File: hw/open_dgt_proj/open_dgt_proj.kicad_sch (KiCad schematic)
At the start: 4 parts, among them SW1 SW_Wuerth_450301014042, U1 MiniF4-STM32F401CEU6

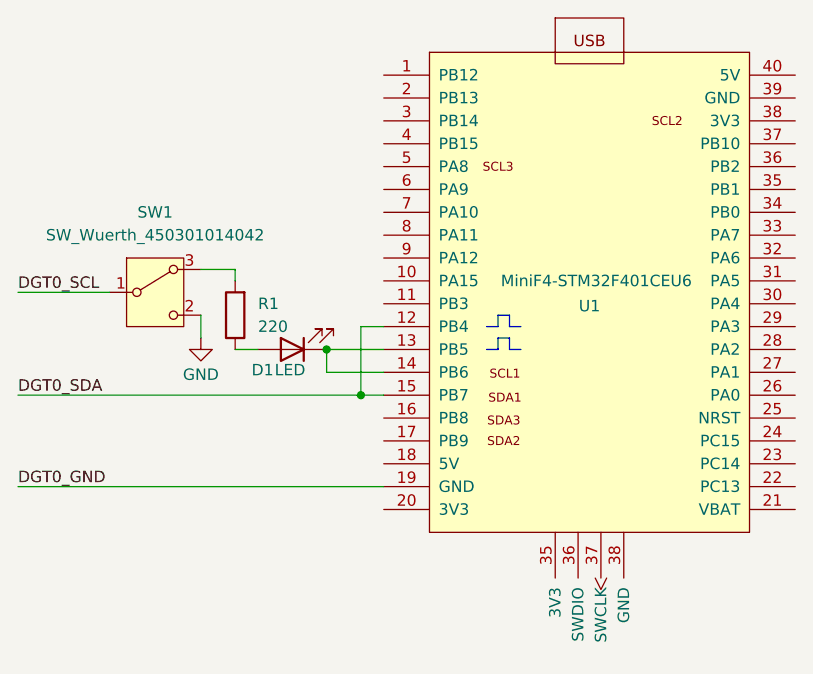
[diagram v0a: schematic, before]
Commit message: Updated project schematic, PCB and 3D model
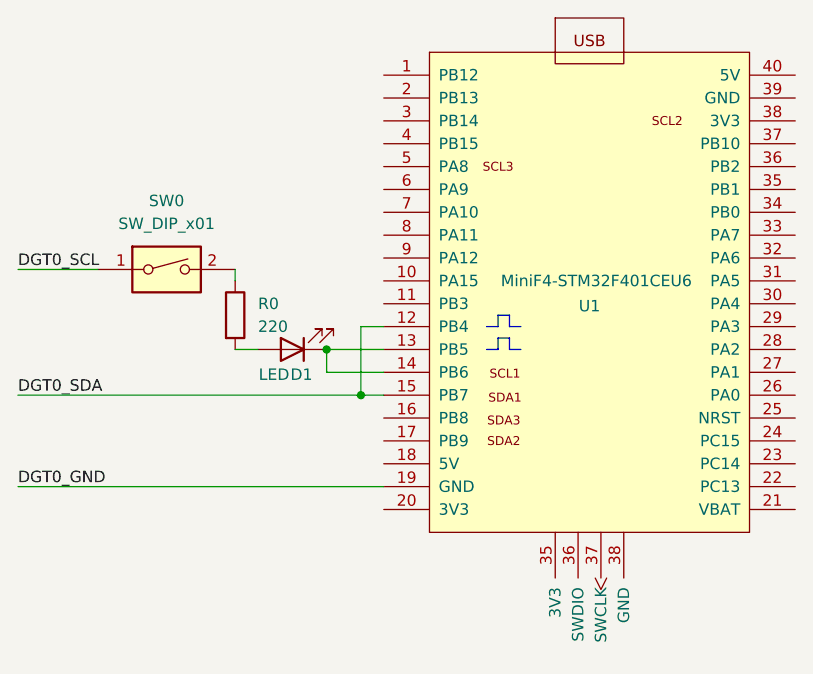
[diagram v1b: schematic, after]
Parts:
- removed R1: 220, symbol Device:R
- removed SW1: SW_Wuerth_450301014042, Button_Switch_THT:SW_Slide-03_Wuerth-WS-SLTV_10x2.5x6.4_P2.54mm, symbol Switch:SW_Wuerth_450301014042
- added R0: 220, Resistor_THT:R_Axial_DIN0207_L6.3mm_D2.5mm_P10.16mm_Horizontal, symbol Device:R
- added SW0: SW_DIP_x01, Button_Switch_THT:SW_DIP_SPSTx01_Slide_6.7x4.1mm_W7.62mm_P2.54mm_LowProfile, symbol Switch:SW_DIP_x01
- D1: footprint (none) -> LED_THT:LED_D5.0mm_FlatTop
- U1: footprint (none) -> BlackPill_v2:YAAJ_BlackPill_SWD_2
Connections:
- net DGT0_SCL: now also SW0.1
- net at D1.2 (A): now also R0.2
- new net: R0.1, SW0.2
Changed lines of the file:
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@@
-	(wire
-		(pts
-			(xy 77.47 83.82) (xy 81.28 83.82)
-		)
-		(stroke
-			(width 0)
-			(type default)
-		)
-	)
 	(wire
 		(pts
@@
 	(wire
 		(pts
-			(xy 77.47 88.9) (xy 77.47 91.44)
-		)
-		(stroke
-			(width 0)
-			(type default)
-		)
-	)
-	(wire
-		(pts
 			(xy 91.44 92.71) (xy 97.79 92.71)
 		)
@@
 	(wire
 		(pts
-			(xy 57.15 86.36) (xy 67.31 86.36)
+			(xy 57.15 83.82) (xy 66.04 83.82)
 		)
 		(stroke
@@
 	)
 	(label "DGT0_SCL"
-		(at 57.15 86.36 0)
+		(at 57.15 83.82 0)
 		(effects
 			(font
@@
 	)
 	(symbol
-		(lib_id "Switch:SW_Wuerth_450301014042")
-		(at 72.39 86.36 0)
+		(lib_id "Device:R")
+		(at 81.28 88.9 0)
 		(unit 1)
 		(exclude_from_sim no)
@@
 		(dnp no)
 		(fields_autoplaced yes)
-		(property "Reference" "SW1"
-			(at 72.39 77.47 0)
-			(effects
-				(font
-					(size 1.27 1.27)
-				)
-			)
-		)
-		(property "Value" "SW_Wuerth_450301014042"
-			(at 72.39 80.01 0)
-			(effects
-				(font
-					(size 1.27 1.27)
-				)
-			)
-		)
-		(property "Footprint" "Button_Switch_THT:SW_Slide-03_Wuerth-WS-SLTV_10x2.5x6.4_P2.54mm"
-			(at 72.39 96.52 0)
-			(effects
-				(font
-					(size 1.27 1.27)
-				)
-				(hide yes)
-			)
-		)
-		(property "Datasheet" "https://www.we-online.com/components/products/datasheet/450301014042.pdf"
-			(at 72.39 93.98 0)
-			(effects
-				(font
-					(size 1.27 1.27)
-				)
-				(hide yes)
-			)
-		)
-		(property "Description" "Switch slide, single pole double throw"
-			(at 72.39 86.36 0)
+		(property "Reference" "R0"
+			(at 83.82 87.6299 0)
+			(effects
+				(font
+					(size 1.27 1.27)
+				)
+				(justify left)
+			)
+		)
+		(property "Value" "220"
+			(at 83.82 90.1699 0)
+			(effects
+				(font
+					(size 1.27 1.27)
+				)
+				(justify left)
+			)
+		)
+		(property "Footprint" "Resistor_THT:R_Axial_DIN0207_L6.3mm_D2.5mm_P10.16mm_Horizontal"
+			(at 79.502 88.9 90)
+			(effects
+				(font
+					(size 1.27 1.27)
+				)
+				(hide yes)
+			)
+		)
+		(property "Datasheet" "~"
+			(at 81.28 88.9 0)
+			(effects
+				(font
+					(size 1.27 1.27)
+				)
+				(hide yes)
+			)
+		)
+		(property "Description" "Resistor"
+			(at 81.28 88.9 0)
 			(effects
 				(font
@@
 		)
 		(pin "2"
-		)
-		(pin "3"
 		)
 		(instances
 			(project ""
 				(path "/c09d2dd6-9539-48f7-8c2c-4fe0c54a0ff8"
-					(reference "SW1")
-					(unit 1)
-				)
-			)
-		)
-	)
-	(symbol
-		(lib_id "power:GND")
-		(at 77.47 91.44 0)
-		(unit 1)
-		(exclude_from_sim no)
-		(in_bom yes)
-		(on_board yes)
-		(dnp no)
-		(property "Reference" "#PWR01"
-			(at 77.47 97.79 0)
-			(effects
-				(font
-					(size 1.27 1.27)
-				)
-				(hide yes)
-			)
-		)
-		(property "Value" "GND"
-			(at 77.47 95.504 0)
-			(effects
-				(font
-					(size 1.27 1.27)
-				)
-			)
-		)
-		(property "Footprint" ""
-			(at 77.47 91.44 0)
-			(effects
-				(font
-					(size 1.27 1.27)
-				)
-				(hide yes)
-			)
-		)
-		(property "Datasheet" ""
-			(at 77.47 91.44 0)
-			(effects
-				(font
-					(size 1.27 1.27)
-				)
-				(hide yes)
-			)
-		)
-		(property "Description" "Power symbol creates a global label with name \"GND\" , ground"
-			(at 77.47 91.44 0)
-			(effects
-				(font
-					(size 1.27 1.27)
-				)
-				(hide yes)
-			)
-		)
-		(pin "1"
-		)
-		(instances
-			(project ""
-				(path "/c09d2dd6-9539-48f7-8c2c-4fe0c54a0ff8"
-					(reference "#PWR01")
+					(reference "R0")
 					(unit 1)
 				)
@@
 			)
 		)
-		(property "Footprint" ""
+		(property "Footprint" "BlackPill_v2:YAAJ_BlackPill_SWD_2"
 			(at 137.16 110.49 0)
 			(effects
@@
 			)
 		)
-		(property "Datasheet" ""
+		(property "Datasheet" "kicad-embed://STM32F411CEU6_Datasheet.pdf"
 			(at 137.16 110.49 0)
 			(effects
@@
 				(path "/c09d2dd6-9539-48f7-8c2c-4fe0c54a0ff8"
 					(reference "U1")
-					(unit 1)
-				)
-			)
-		)
-	)
-	(symbol
-		(lib_id "Device:R")
-		(at 81.28 88.9 180)
-		(unit 1)
-		(exclude_from_sim no)
-		(in_bom yes)
-		(on_board yes)
-		(dnp no)
-		(fields_autoplaced yes)
-		(property "Reference" "R1"
-			(at 83.82 87.6299 0)
-			(effects
-				(font
-					(size 1.27 1.27)
-				)
-				(justify right)
-			)
-		)
-		(property "Value" "220"
-			(at 83.82 90.1699 0)
-			(effects
-				(font
-					(size 1.27 1.27)
-				)
-				(justify right)
-			)
-		)
-		(property "Footprint" ""
-			(at 83.058 88.9 90)
-			(effects
-				(font
-					(size 1.27 1.27)
-				)
-				(hide yes)
-			)
-		)
-		(property "Datasheet" "~"
-			(at 81.28 88.9 0)
-			(effects
-				(font
-					(size 1.27 1.27)
-				)
-				(hide yes)
-			)
-		)
-		(property "Description" "Resistor"
-			(at 81.28 88.9 0)
-			(effects
-				(font
-					(size 1.27 1.27)
-				)
-				(hide yes)
-			)
-		)
-		(pin "2"
-		)
-		(pin "1"
-		)
-		(instances
-			(project ""
-				(path "/c09d2dd6-9539-48f7-8c2c-4fe0c54a0ff8"
-					(reference "R1")
 					(unit 1)
 				)
@@
 		(dnp no)
 		(property "Reference" "D1"
-			(at 84.328 94.996 0)
+			(at 88.646 95.504 0)
 			(effects
 				(font
@@
 		)
 		(property "Value" "LED"
-			(at 87.376 94.996 0)
-			(effects
-				(font
-					(size 1.27 1.27)
-				)
-			)
-		)
-		(property "Footprint" ""
+			(at 85.598 95.504 0)
+			(effects
+				(font
+					(size 1.27 1.27)
+				)
+			)
+		)
+		(property "Footprint" "LED_THT:LED_D5.0mm_FlatTop"
 			(at 87.63 92.71 0)
 			(effects
@@
 					(unit 1)
 				)
+			)
+		)
+	)
+	(symbol
+		(lib_id "Switch:SW_DIP_x01")
+		(at 73.66 83.82 0)
+		(unit 1)
+		(exclude_from_sim no)
+		(in_bom yes)
+		(on_board yes)
+		(dnp no)
+		(fields_autoplaced yes)
+		(property "Reference" "SW0"
+			(at 73.66 76.2 0)
+			(effects
+				(font
+					(size 1.27 1.27)
+				)
+			)
+		)
+		(property "Value" "SW_DIP_x01"
+			(at 73.66 78.74 0)
+			(effects
+				(font
+					(size 1.27 1.27)
+				)
+			)
+		)
+		(property "Footprint" "Button_Switch_THT:SW_DIP_SPSTx01_Slide_6.7x4.1mm_W7.62mm_P2.54mm_LowProfile"
+			(at 73.66 83.82 0)
+			(effects
+				(font
+					(size 1.27 1.27)
+				)
+				(hide yes)
+			)
+		)
+		(property "Datasheet" "~"
+			(at 73.66 83.82 0)
+			(effects
+				(font
+					(size 1.27 1.27)
+				)
+				(hide yes)
+			)
+		)
+		(property "Description" "1x DIP Switch, Single Pole Single Throw (SPST) switch, small symbol"
+			(at 73.66 83.82 0)
+			(effects
+				(font
+					(size 1.27 1.27)
+				)
+				(hide yes)
+			)
+		)
+		(pin "2"
+		)
+		(pin "1"
+		)
+		(instances
+			(project ""
+				(path "/c09d2dd6-9539-48f7-8c2c-4fe0c54a0ff8"
+					(reference "SW0")
+					(unit 1)
+				)
